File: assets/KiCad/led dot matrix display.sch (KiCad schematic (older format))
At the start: 0 parts

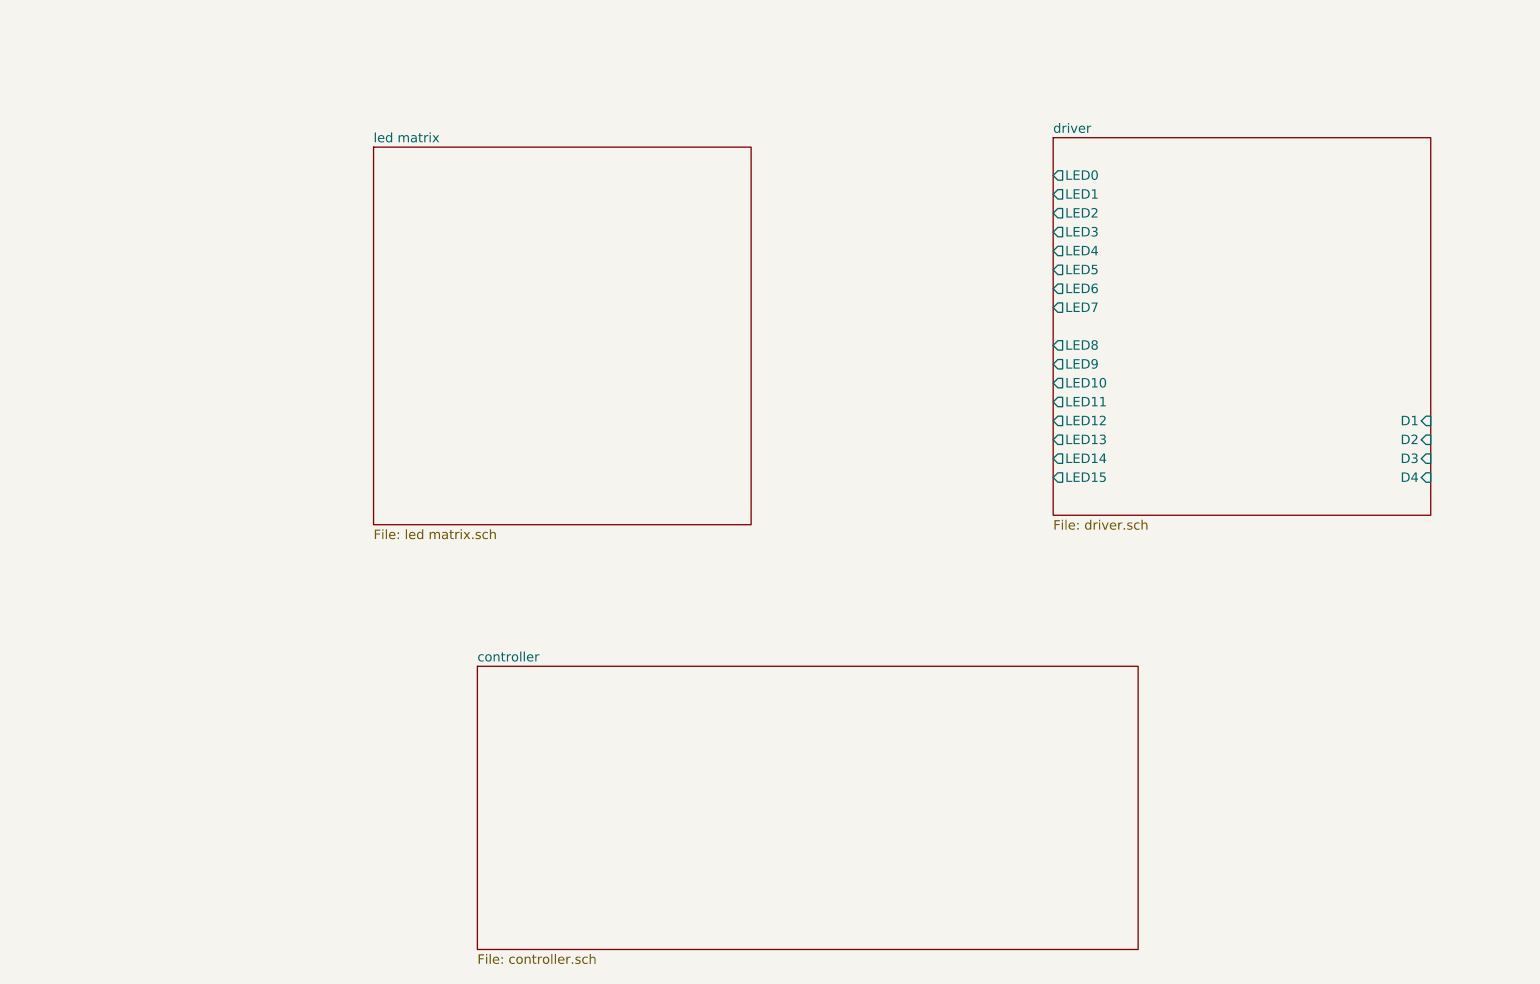
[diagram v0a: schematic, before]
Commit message: minor update
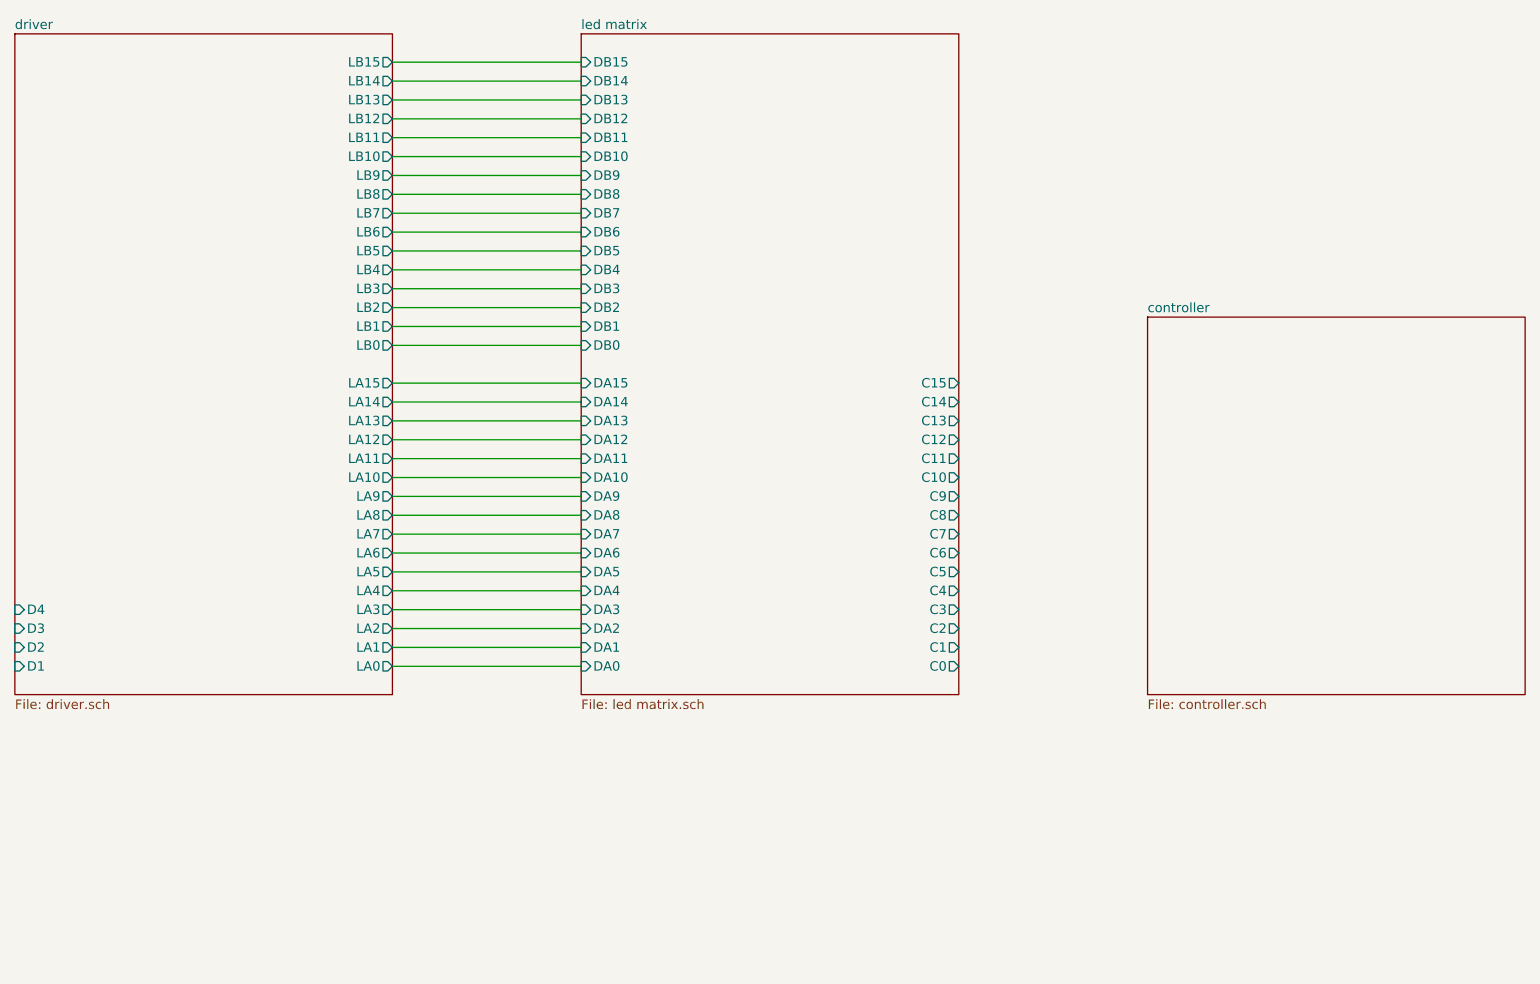
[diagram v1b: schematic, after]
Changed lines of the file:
@@
 $Descr A4 11693 8268
 encoding utf-8
-Sheet 1 5
+Sheet 1 8
 Title "test"
 Date ""
@@
 $EndDescr
 $Sheet
-S 7350 1550 2000 2000
-U 5F5984FE
-F0 "driver" 50
-F1 "driver.sch" 50
-F2 "D1" I R 9350 3050 50
-F3 "D2" I R 9350 3150 50
-F4 "D3" I R 9350 3250 50
-F5 "D4" I R 9350 3350 50
-F6 "LED0" O L 7350 1750 50
-F7 "LED1" O L 7350 1850 50
-F8 "LED2" O L 7350 1950 50
-F9 "LED3" O L 7350 2050 50
-F10 "LED4" O L 7350 2150 50
-F11 "LED5" O L 7350 2250 50
-F12 "LED6" O L 7350 2350 50
-F13 "LED7" O L 7350 2450 50
-F14 "LED8" O L 7350 2650 50
-F15 "LED9" O L 7350 2750 50
-F16 "LED10" O L 7350 2850 50
-F17 "LED11" O L 7350 2950 50
-F18 "LED12" O L 7350 3050 50
-F19 "LED13" O L 7350 3150 50
-F20 "LED14" O L 7350 3250 50
-F21 "LED15" O L 7350 3350 50
+S 4850 1000 2000 3500
+U 5F54EEE0
+F0 "led matrix" 50
+F1 "led matrix.sch" 50
+F2 "C0" O R 6850 4350 50
+F3 "C1" O R 6850 4250 50
+F4 "C2" O R 6850 4150 50
+F5 "C3" O R 6850 4050 50
+F6 "C4" O R 6850 3950 50
+F7 "C5" O R 6850 3850 50
+F8 "C6" O R 6850 3750 50
+F9 "C7" O R 6850 3650 50
+F10 "C8" O R 6850 3550 50
+F11 "C9" O R 6850 3450 50
+F12 "C10" O R 6850 3350 50
+F13 "C11" O R 6850 3250 50
+F14 "C12" O R 6850 3150 50
+F15 "C13" O R 6850 3050 50
+F16 "C14" O R 6850 2950 50
+F17 "C15" O R 6850 2850 50
+F18 "DA0" I L 4850 4350 50
+F19 "DA1" I L 4850 4250 50
+F20 "DA2" I L 4850 4150 50
+F21 "DA3" I L 4850 4050 50
+F22 "DA4" I L 4850 3950 50
+F23 "DA5" I L 4850 3850 50
+F24 "DA6" I L 4850 3750 50
+F25 "DA7" I L 4850 3650 50
+F26 "DB0" I L 4850 2650 50
+F27 "DB1" I L 4850 2550 50
+F28 "DB2" I L 4850 2450 50
+F29 "DB3" I L 4850 2350 50
+F30 "DB4" I L 4850 2250 50
+F31 "DB5" I L 4850 2150 50
+F32 "DB6" I L 4850 2050 50
+F33 "DB7" I L 4850 1950 50
+F34 "DA8" I L 4850 3550 50
+F35 "DA9" I L 4850 3450 50
+F36 "DA10" I L 4850 3350 50
+F37 "DA11" I L 4850 3250 50
+F38 "DA12" I L 4850 3150 50
+F39 "DA13" I L 4850 3050 50
+F40 "DA14" I L 4850 2950 50
+F41 "DA15" I L 4850 2850 50
+F42 "DB8" I L 4850 1850 50
+F43 "DB9" I L 4850 1750 50
+F44 "DB10" I L 4850 1650 50
+F45 "DB11" I L 4850 1550 50
+F46 "DB12" I L 4850 1450 50
+F47 "DB13" I L 4850 1350 50
+F48 "DB14" I L 4850 1250 50
+F49 "DB15" I L 4850 1150 50
 $EndSheet
 $Sheet
-S 4300 4350 3500 1500
-U 5F5AB140
+S 7850 2500 2000 2000
+U 5F5A0E48
 F0 "controller" 50
 F1 "controller.sch" 50
 $EndSheet
 $Sheet
-S 3750 1600 2000 2000
-U 5F54EEE0
-F0 "led matrix" 50
-F1 "led matrix.sch" 50
+S 1850 1000 2000 3500
+U 5F5984FE
+F0 "driver" 50
+F1 "driver.sch" 50
+F2 "D1" I L 1850 4350 50
+F3 "D2" I L 1850 4250 50
+F4 "D3" I L 1850 4150 50
+F5 "D4" I L 1850 4050 50
+F6 "LA0" O R 3850 4350 50
+F7 "LA1" O R 3850 4250 50
+F8 "LA2" O R 3850 4150 50
+F9 "LA3" O R 3850 4050 50
+F10 "LA4" O R 3850 3950 50
+F11 "LA5" O R 3850 3850 50
+F12 "LA6" O R 3850 3750 50
+F13 "LA7" O R 3850 3650 50
+F14 "LA8" O R 3850 3550 50
+F15 "LA9" O R 3850 3450 50
+F16 "LA10" O R 3850 3350 50
+F17 "LA11" O R 3850 3250 50
+F18 "LA12" O R 3850 3150 50
+F19 "LA13" O R 3850 3050 50
+F20 "LA14" O R 3850 2950 50
+F21 "LA15" O R 3850 2850 50
+F22 "LB0" O R 3850 2650 50
+F23 "LB1" O R 3850 2550 50
+F24 "LB2" O R 3850 2450 50
+F25 "LB3" O R 3850 2350 50
+F26 "LB4" O R 3850 2250 50
+F27 "LB5" O R 3850 2150 50
+F28 "LB6" O R 3850 2050 50
+F29 "LB7" O R 3850 1950 50
+F30 "LB8" O R 3850 1850 50
+F31 "LB9" O R 3850 1750 50
+F32 "LB10" O R 3850 1650 50
+F33 "LB11" O R 3850 1550 50
+F34 "LB12" O R 3850 1450 50
+F35 "LB13" O R 3850 1350 50
+F36 "LB14" O R 3850 1250 50
+F37 "LB15" O R 3850 1150 50
 $EndSheet
+Wire Wire Line
+	3850 4350 4850 4350
+Wire Wire Line
+	3850 4250 4850 4250
+Wire Wire Line
+	3850 4150 4850 4150
+Wire Wire Line
+	3850 4050 4850 4050
+Wire Wire Line
+	3850 3950 4850 3950
+Wire Wire Line
+	3850 3850 4850 3850
+Wire Wire Line
+	3850 3750 4850 3750
+Wire Wire Line
+	3850 3650 4850 3650
+Wire Wire Line
+	3850 3550 4850 3550
+Wire Wire Line
+	3850 3450 4850 3450
+Wire Wire Line
+	3850 3350 4850 3350
+Wire Wire Line
+	3850 3250 4850 3250
+Wire Wire Line
+	3850 3150 4850 3150
+Wire Wire Line
+	3850 3050 4850 3050
+Wire Wire Line
+	3850 2950 4850 2950
+Wire Wire Line
+	3850 2850 4850 2850
+Wire Wire Line
+	3850 2650 4850 2650
+Wire Wire Line
+	3850 2550 4850 2550
+Wire Wire Line
+	3850 2450 4850 2450
+Wire Wire Line
+	3850 2350 4850 2350
+Wire Wire Line
+	3850 2250 4850 2250
+Wire Wire Line
+	3850 2150 4850 2150
+Wire Wire Line
+	3850 2050 4850 2050
+Wire Wire Line
+	3850 1950 4850 1950
+Wire Wire Line
+	3850 1850 4850 1850
+Wire Wire Line
+	3850 1750 4850 1750
+Wire Wire Line
+	3850 1650 4850 1650
+Wire Wire Line
+	3850 1550 4850 1550
+Wire Wire Line
+	3850 1450 4850 1450
+Wire Wire Line
+	3850 1350 4850 1350
+Wire Wire Line
+	3850 1250 4850 1250
+Wire Wire Line
+	3850 1150 4850 1150
 $EndSCHEMATC
